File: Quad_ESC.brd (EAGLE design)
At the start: 96.5 x 39.9 mm, 28 parts, among them Y1 ECS-80-S-4X

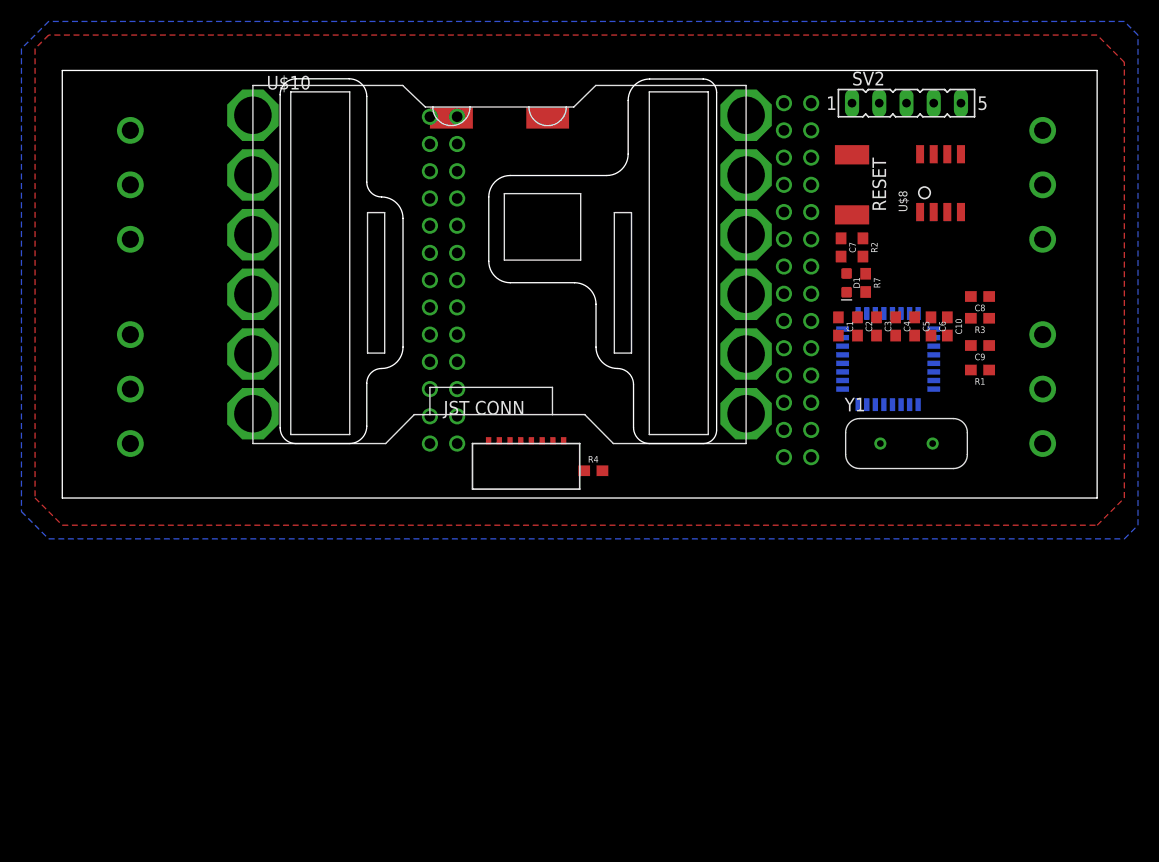
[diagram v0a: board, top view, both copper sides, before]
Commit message: Update Quad_ESC.brd
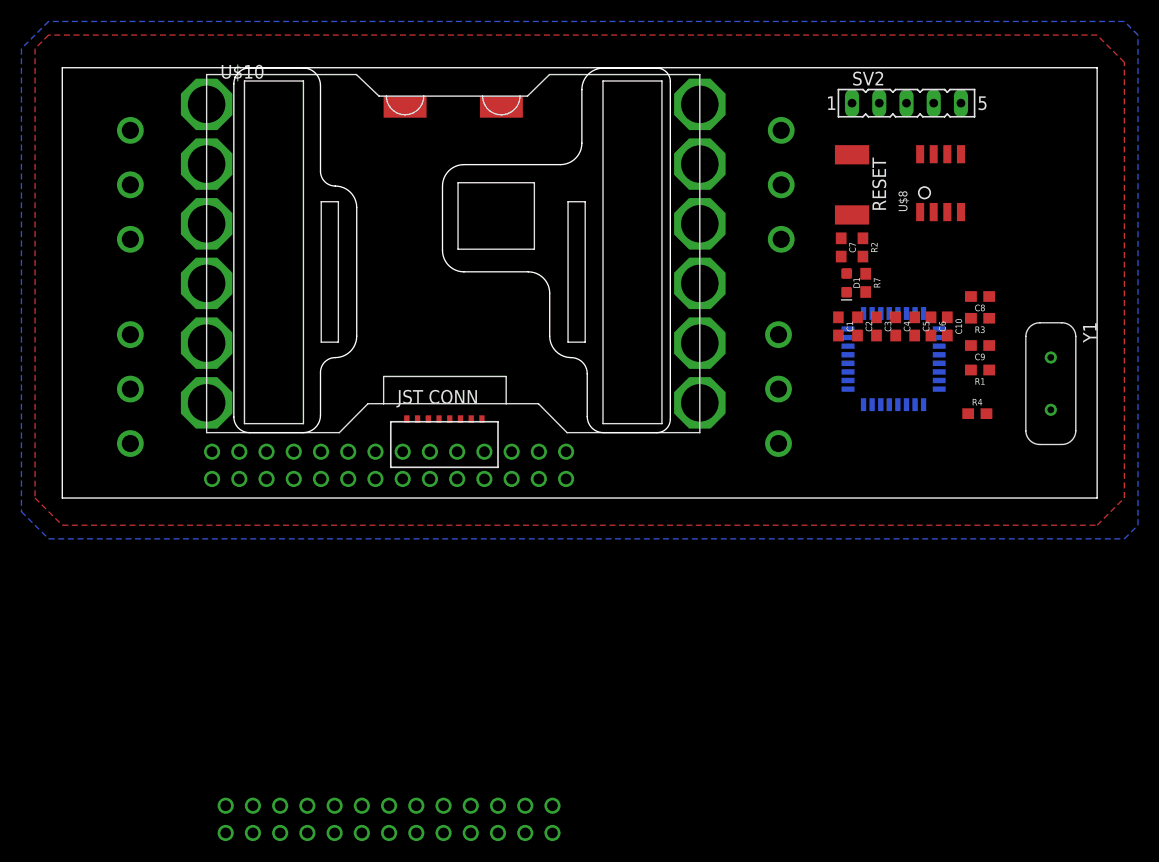
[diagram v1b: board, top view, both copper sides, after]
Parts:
- moved U$2 64.2 mm to (14.0, 3.05), turned to 180 degrees
- moved R4 36.2 mm to (85.3, 7.87)
- moved U$7 24.6 mm to (66.8, 10.2)
- moved U$6 24.4 mm to (67.1, 29.2)
- moved Y1 14.6 mm to (92.2, 10.7), turned to 270 degrees
- moved U$9 7.89 mm to (40.6, 7.11)
- moved U$10 4.44 mm to (13.5, 6.10)
- moved U$4 0.51 mm to (81.8, 10.2)
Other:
- board size 96.5 x 39.9 mm -> 96.5 x 40.1 mm
